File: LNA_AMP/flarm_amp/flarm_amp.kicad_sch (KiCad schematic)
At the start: 40 parts, among them J1 ANT, J2 OUT, Q1 BC817, Q2 IRLML2060, U1 PGA-105, U2 LM78L05_SO8

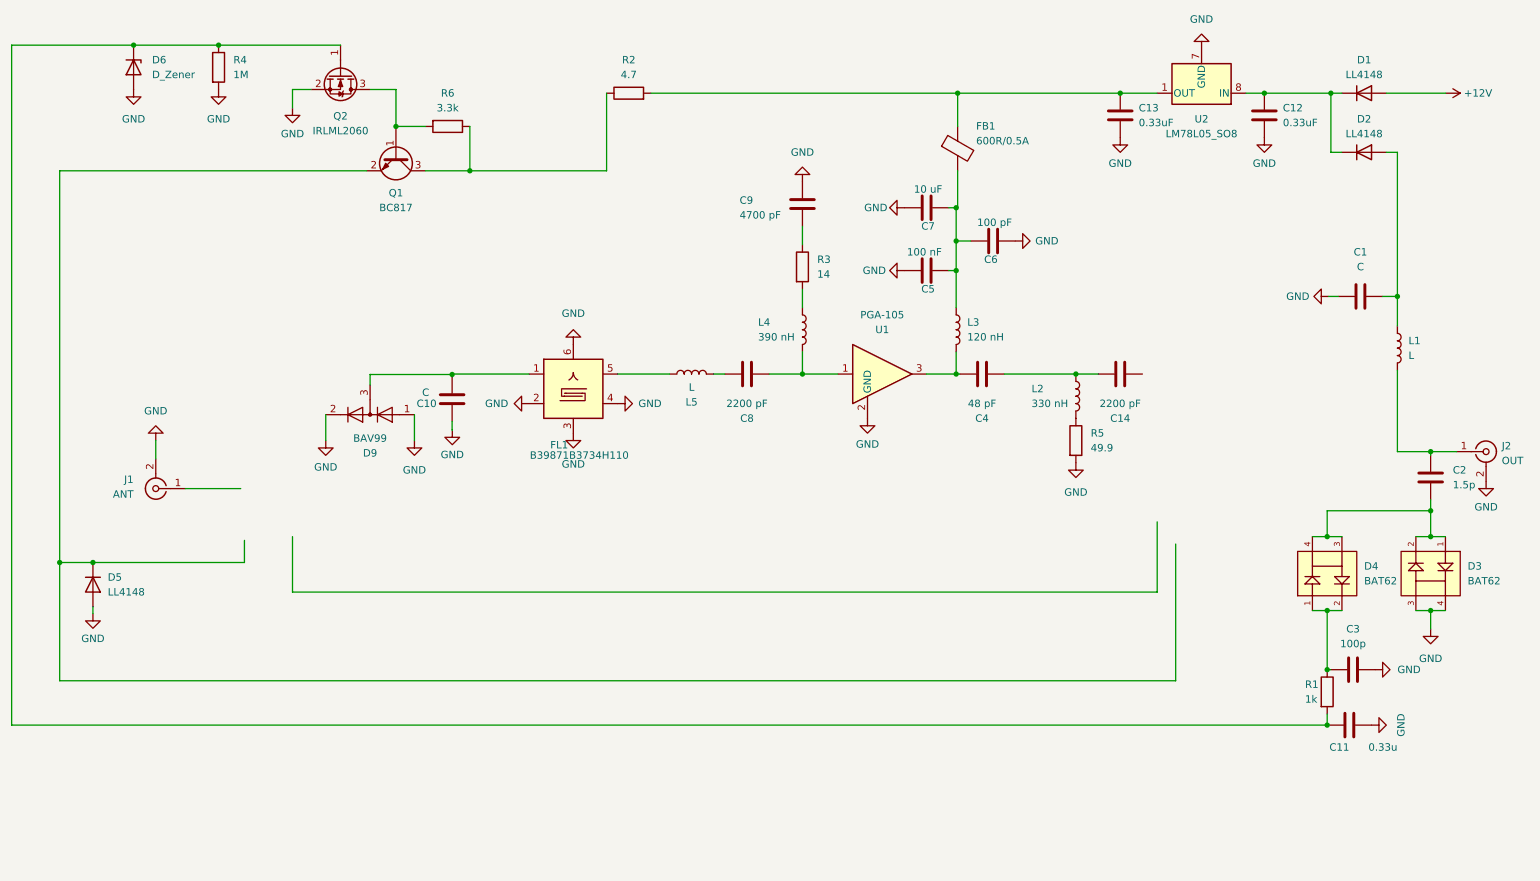
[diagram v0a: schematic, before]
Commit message: friggi scemo
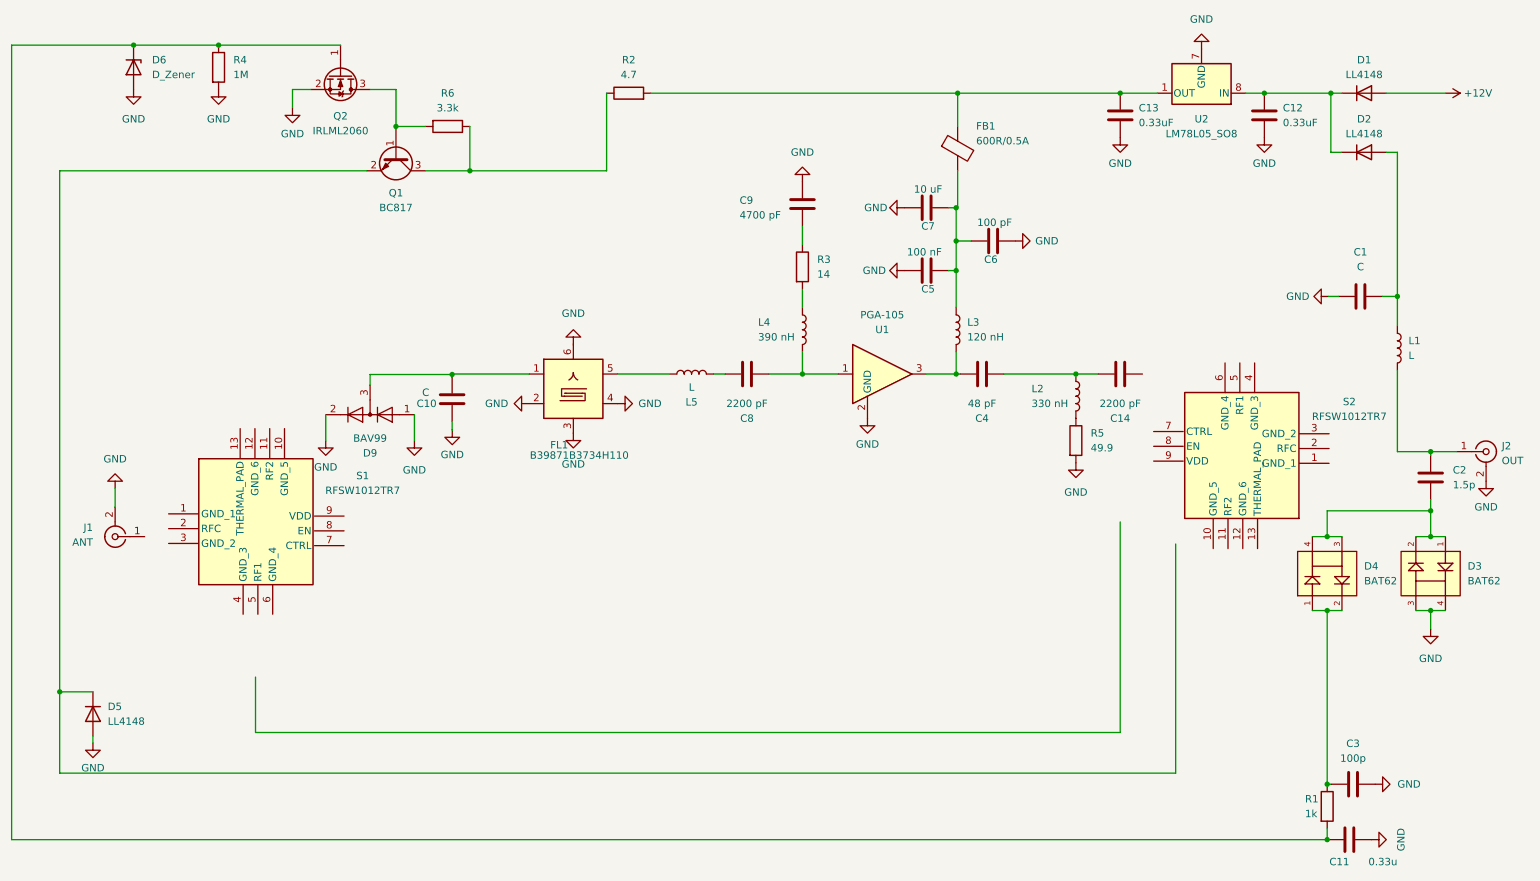
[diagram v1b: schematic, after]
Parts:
- added S1, S2: RFSW1012TR7, QFN50P200X200X60-13N-D, symbol My_Library:RFSW1012TR7
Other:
- moved on the sheet: C11, C3, D5, J1, R1
